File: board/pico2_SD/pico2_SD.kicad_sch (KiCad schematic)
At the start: 3 parts, among them J1 USB_C_Receptacle_USB2.0, J2 SD_Card, U1 RP2040

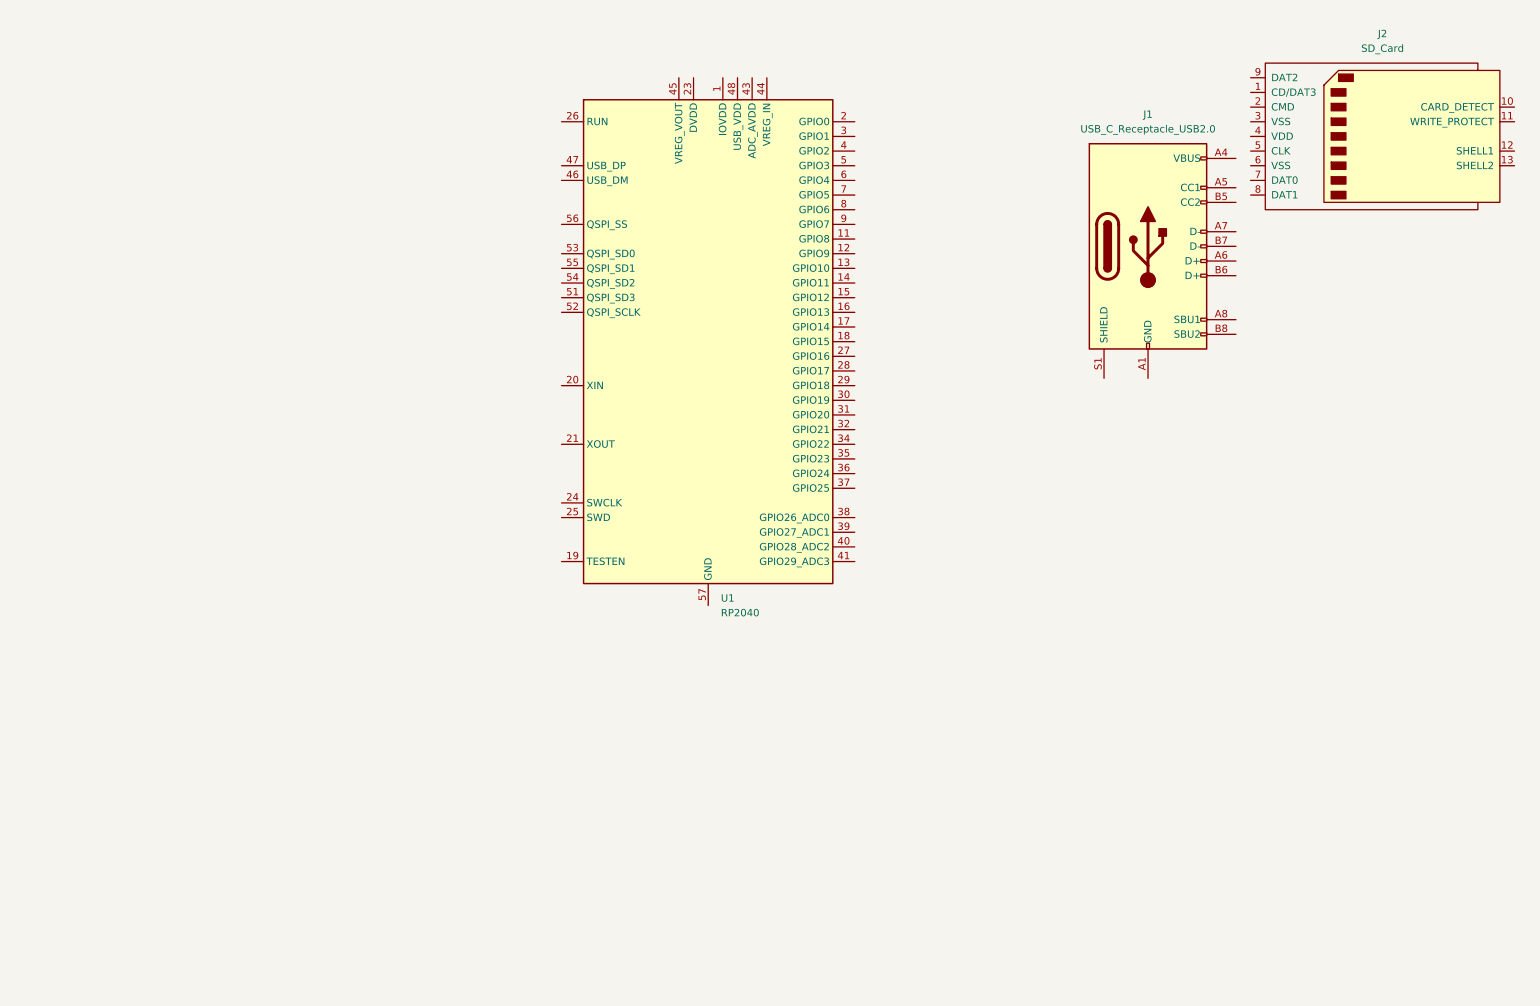
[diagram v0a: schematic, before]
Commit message: start schimatic
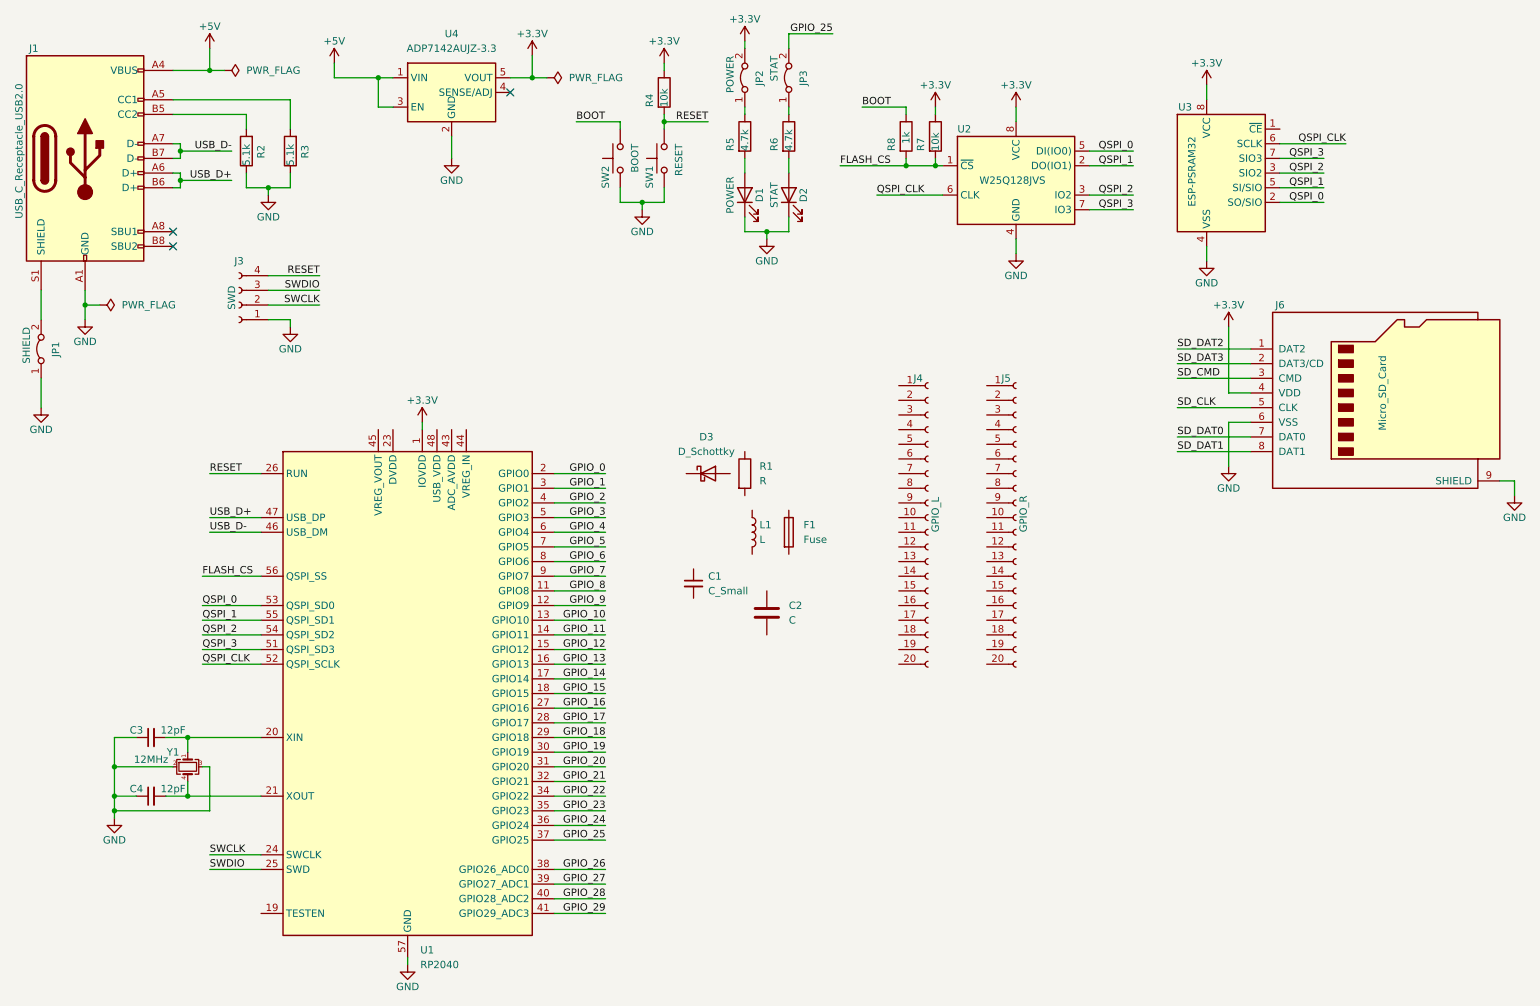
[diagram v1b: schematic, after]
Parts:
- removed J2: SD_Card, symbol Connector:SD_Card
- added C1: C_Small, symbol Device:C_Small
- added C2: C, symbol Device:C
- added C3, C4: 12pF, symbol Device:C_Small
- added D1: POWER, symbol Device:LED
- added D2: STAT, symbol Device:LED
- added D3: D_Schottky, symbol Device:D_Schottky
- added F1: Fuse, symbol Device:Fuse
- added J3: SWD, symbol Connector:Conn_01x04_Female
- added J4: GPIO_L, symbol Connector:Conn_01x20_Female
- added J5: GPIO_R, symbol Connector:Conn_01x20_Female
- added J6: Micro_SD_Card, symbol Connector:Micro_SD_Card
- added JP1: SHIELD, symbol Jumper:Jumper_2_Bridged
- added JP2: POWER, symbol Jumper:Jumper_2_Bridged
- added JP3: STAT, symbol Jumper:Jumper_2_Bridged
- added L1: L, symbol Device:L
- added R1: R, symbol Device:R
- added R2, R3: 5.1k, symbol Device:R
- added R4, R7: 10k, symbol Device:R
- added R5, R6: 4.7k, symbol Device:R
- added R8: 1k, symbol Device:R
- added SW1: RESET, symbol Switch:SW_Push
- added SW2: BOOT, symbol Switch:SW_Push
- added U2: W25Q128JVS, Package_SO:SOIC-8_5.23x5.23mm_P1.27mm, symbol Memory_Flash:W25Q128JVS
- added U3: ESP-PSRAM32, Package_SO:SOIC-8_3.9x4.9mm_P1.27mm, symbol Memory_RAM:ESP-PSRAM32
- added U4: ADP7142AUJZ-3.3, Package_TO_SOT_SMD:TSOT-23-5, symbol Regulator_Linear:ADP7142AUJZ-3.3
- added Y1: 12MHz, symbol Device:Crystal_GND23_Small
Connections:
- net GND: now reaches J1.A1 (GND), J1.A12 (GND), J1.B1 (GND), J1.B12 (GND)
- net GND: now also U1.57 (GND), C3.1, C4.1, D1.1 (K), D2.1 (K), J3.1 (Pin_1), J6.6 (VSS), J6.9 (SHIELD), JP1.1 (A), R2.1, R3.1, SW1.1, SW2.1, U2.4 (GND), U3.4 (VSS), U4.2 (GND), Y1.2, Y1.3
- net +5V: now reaches J1.A4 (VBUS), J1.A9 (VBUS), J1.B4 (VBUS), J1.B9 (VBUS)
- net +5V: now also U4.1 (VIN), U4.3 (EN)
- net at J1.A5 (CC1): now also R3.2
- net USB_D+: now reaches J1.A6 (D+)
- net USB_D+: now also J1.B6 (D+), U1.47 (USB_DP)
- net USB_D-: now reaches J1.A7 (D-)
- net USB_D-: now also J1.B7 (D-), U1.46 (USB_DM)
- net at J1.B5 (CC2): now also R2.2
- net at J1.S1 (SHIELD): now also JP1.2 (B)
- net +3.3V: now reaches U1.1 (IOVDD), U1.10 (IOVDD), U1.22 (IOVDD), U1.33 (IOVDD), U1.42 (IOVDD), U1.49 (IOVDD)
- net +3.3V: now also J6.4 (VDD), JP2.2 (B), R4.1, R7.1, U2.8 (VCC), U3.8 (VCC), U4.5 (VOUT)
- net GPIO_8: now reaches U1.11 (GPIO8)
- net GPIO_9: now reaches U1.12 (GPIO9)
- net GPIO_10: now reaches U1.13 (GPIO10)
- net GPIO_11: now reaches U1.14 (GPIO11)
- net GPIO_12: now reaches U1.15 (GPIO12)
- net GPIO_13: now reaches U1.16 (GPIO13)
- net GPIO_14: now reaches U1.17 (GPIO14)
- net GPIO_15: now reaches U1.18 (GPIO15)
- net GPIO_0: now reaches U1.2 (GPIO0)
- net at U1.20 (XIN): now also C3.2, Y1.1
- net at U1.21 (XOUT): now also C4.2, Y1.4
- net SWCLK: now reaches U1.24 (SWCLK)
- net SWCLK: now also J3.2 (Pin_2)
- net SWDIO: now reaches U1.25 (SWD)
- net SWDIO: now also J3.3 (Pin_3)
- net RESET: now reaches U1.26 (RUN)
- net RESET: now also J3.4 (Pin_4), R4.2, SW1.2
- net GPIO_16: now reaches U1.27 (GPIO16)
- net GPIO_17: now reaches U1.28 (GPIO17)
- net GPIO_18: now reaches U1.29 (GPIO18)
- net GPIO_1: now reaches U1.3 (GPIO1)
- net GPIO_19: now reaches U1.30 (GPIO19)
- net GPIO_20: now reaches U1.31 (GPIO20)
- net GPIO_21: now reaches U1.32 (GPIO21)
- net GPIO_22: now reaches U1.34 (GPIO22)
- net GPIO_23: now reaches U1.35 (GPIO23)
- net GPIO_24: now reaches U1.36 (GPIO24)
- net GPIO_25: now reaches U1.37 (GPIO25)
- net GPIO_25: now also JP3.2 (B)
- net GPIO_26: now reaches U1.38 (GPIO26_ADC0)
- net GPIO_27: now reaches U1.39 (GPIO27_ADC1)
- net GPIO_2: now reaches U1.4 (GPIO2)
- net GPIO_28: now reaches U1.40 (GPIO28_ADC2)
- net GPIO_29: now reaches U1.41 (GPIO29_ADC3)
- net GPIO_3: now reaches U1.5 (GPIO3)
- net QSPI_3: now reaches U1.51 (QSPI_SD3)
- net QSPI_3: now also U2.7 (IO3), U3.7 (SIO3)
- net QSPI_CLK: now reaches U1.52 (QSPI_SCLK)
- net QSPI_CLK: now also U2.6 (CLK), U3.6 (SCLK)
- net QSPI_0: now reaches U1.53 (QSPI_SD0)
- net QSPI_0: now also U2.5 (DI(IO0)), U3.2 (SO/SIO)
- net QSPI_2: now reaches U1.54 (QSPI_SD2)
- net QSPI_2: now also U2.3 (IO2), U3.3 (SIO2)
- net QSPI_1: now reaches U1.55 (QSPI_SD1)
- net QSPI_1: now also U2.2 (DO(IO1)), U3.5 (SI/SIO)
- net FLASH_CS: now reaches U1.56 (QSPI_SS)
- net FLASH_CS: now also R7.2, R8.2, U2.1 (~{CS})
- net GPIO_4: now reaches U1.6 (GPIO4)
- net GPIO_5: now reaches U1.7 (GPIO5)
- net GPIO_6: now reaches U1.8 (GPIO6)
- net GPIO_7: now reaches U1.9 (GPIO7)
- new net: JP3.1 (A), R6.1
- new net: D2.2 (A), R6.2
- new net: JP2.1 (A), R5.1
- new net: D1.2 (A), R5.2
- new net BOOT: R8.1, SW2.2
- new net SD_CLK: J6.5 (CLK)
- new net SD_CMD: J6.3 (CMD)
- new net SD_DAT0: J6.7 (DAT0)
- new net SD_DAT1: J6.8 (DAT1)
- new net SD_DAT2: J6.1 (DAT2)
- new net SD_DAT3: J6.2 (DAT3/CD)
- no-connect marks 0 -> 3
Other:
- moved on the sheet: J1, U1
